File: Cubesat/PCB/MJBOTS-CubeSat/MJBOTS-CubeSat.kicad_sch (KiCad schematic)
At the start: 19 parts, among them J1 Display, J10 MOTOR3-XT30, J12 MOTOR3, J2 MPU 6050, J3 Pi_GPIO, J4 CAN, J5 MOTOR1, J6 MOTOR2, J7 INPUT-XT60, J8 MOTOR1-XT30, J9 MOTOR2-XT30, U1 LM2596S

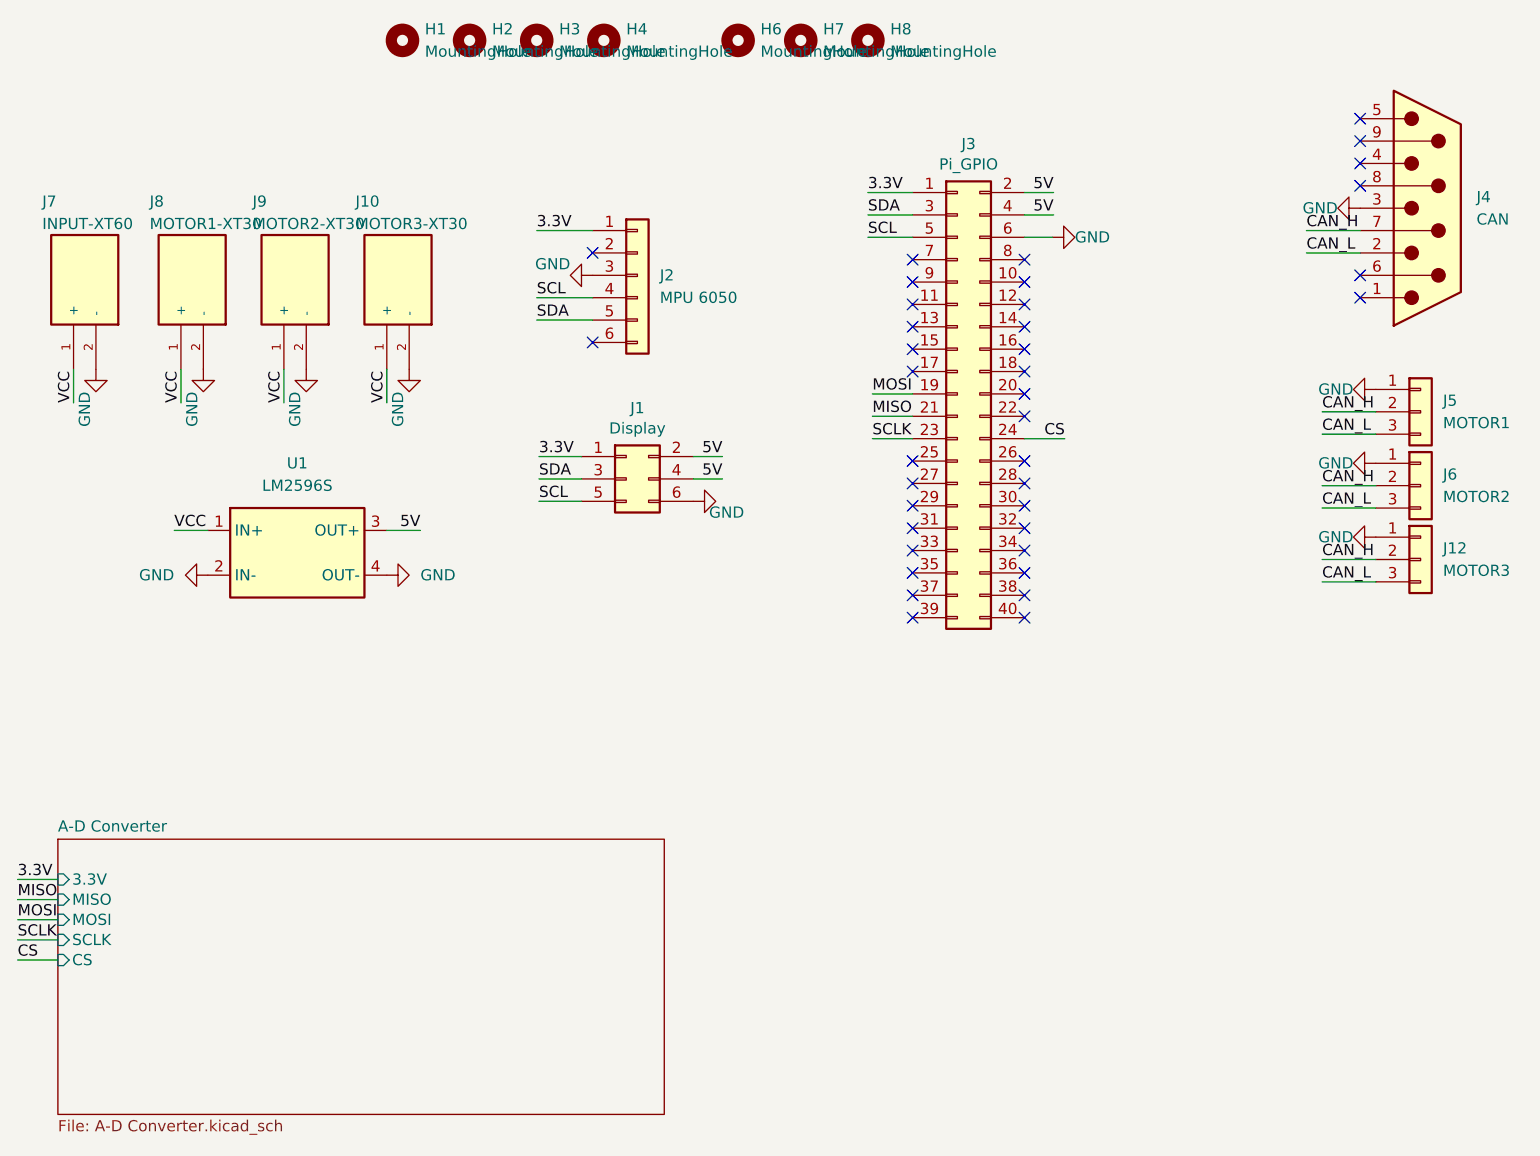
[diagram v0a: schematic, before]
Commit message: Final Updates "HOPEFULLY"
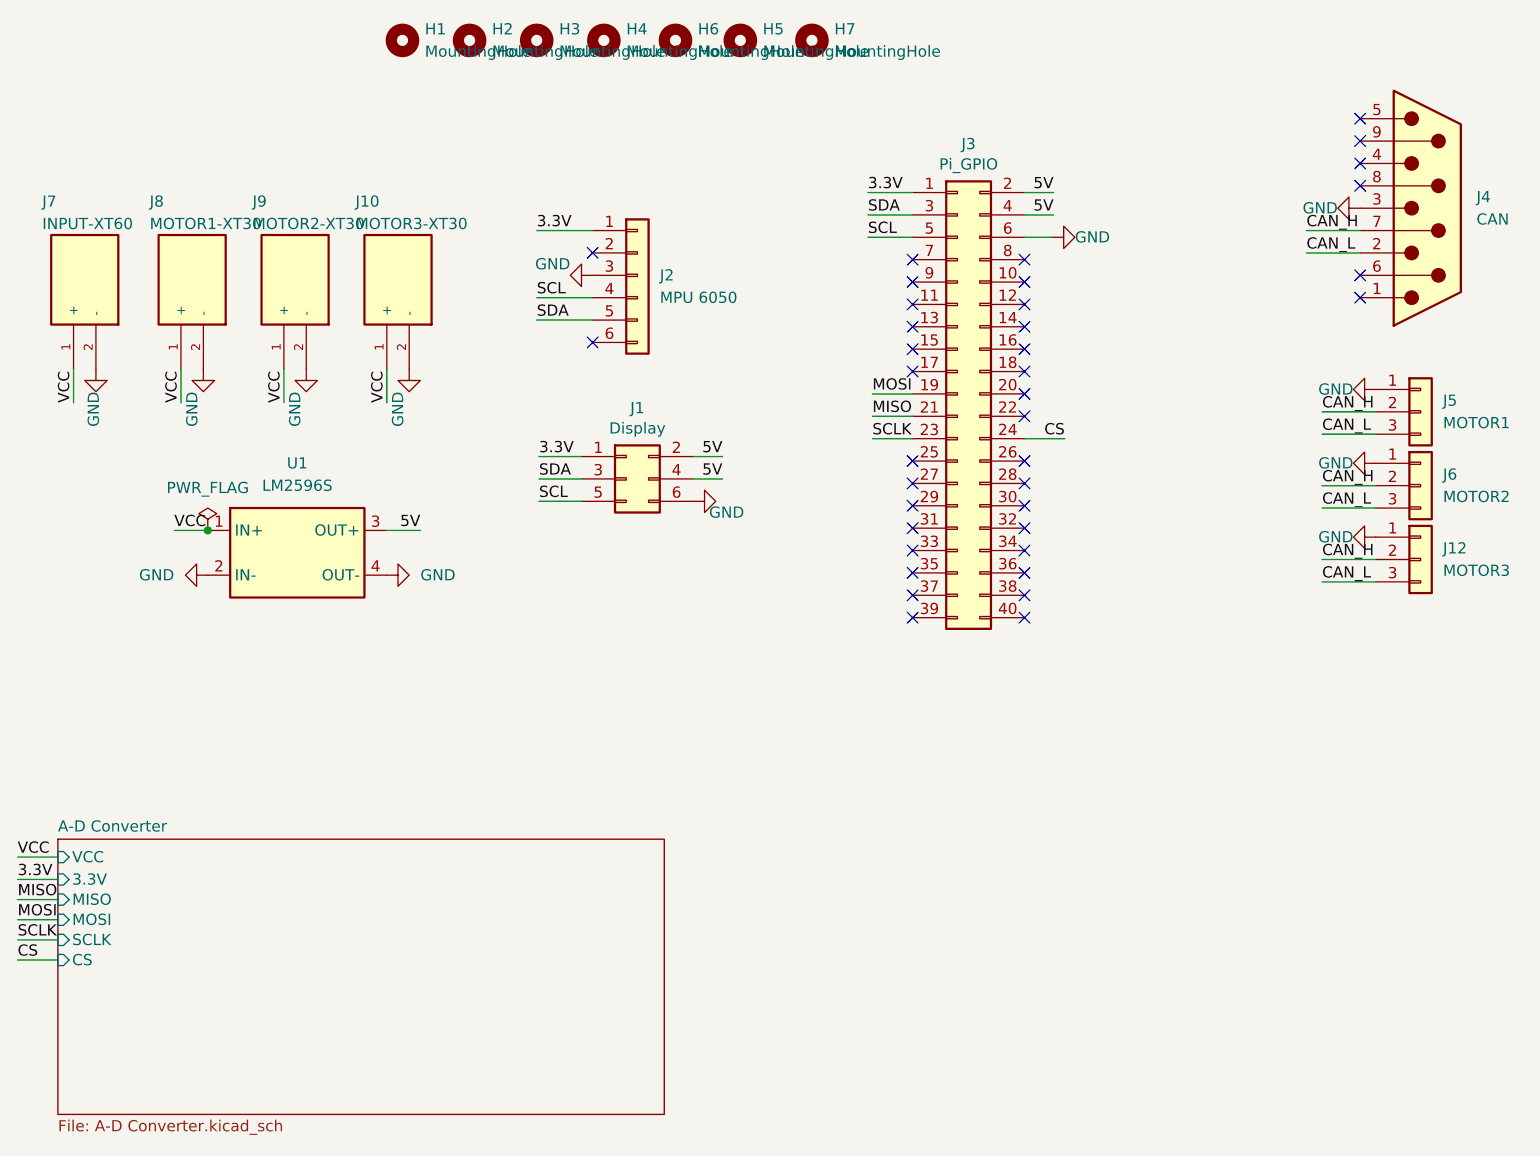
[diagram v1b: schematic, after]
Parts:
- removed H8: MountingHole, MountingHole:MountingHole_2.5mm, symbol Mechanical:MountingHole
- added H5: MountingHole, MountingHole:MountingHole_2.5mm, symbol Mechanical:MountingHole
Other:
- sheet A-D Converter ports: added VCC; removed none
- moved on the sheet: H6
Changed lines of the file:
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@@
 (kicad_sch (version 20211123) (generator eeschema)
   (paper "A4")
+  (junction (at 76.962 96.266) (diameter 0) (color 0 0 0 0)
+  )
   (no_connect (at 156.972 98.552))
   (no_connect (at 156.972 65.532))
@@
     (stroke (width 0) (type default) (color 0 0 0 0))
   )
+  (wire (pts (xy 55.372 133.35) (xy 59.944 133.35))
+    (stroke (width 0) (type default) (color 0 0 0 0))
+  )
   (wire (pts (xy 151.892 60.452) (xy 156.972 60.452))
     (stroke (width 0) (type default) (color 0 0 0 0))
@@
     (effects (font (size 1.27 1.27)) (justify left bottom))
   )
+  (label "VCC" (at 55.372 133.35 0)
+    (effects (font (size 1.27 1.27)) (justify left bottom))
+  )
   (label "5V" (at 135.382 90.424 180)
     (effects (font (size 1.27 1.27)) (justify right bottom))
@@
     (effects (font (size 1.27 1.27)) (justify left bottom))
   )
-  (symbol (lib_id "Mechanical:MountingHole") (at 137.16 40.64 0) (unit 1)
-    (in_bom yes) (on_board yes) (fields_autoplaced)
-    (property "Reference" "H6" (id 0) (at 139.7 39.3699 0)
-      (effects (font (size 1.27 1.27)) (justify left))
-    )
-    (property "Value" "MountingHole" (id 1) (at 139.7 41.9099 0)
-      (effects (font (size 1.27 1.27)) (justify left))
-    )
-    (property "Footprint" "MountingHole:MountingHole_2.5mm" (id 2) (at 137.16 40.64 0)
-      (effects (font (size 1.27 1.27)) hide)
-    )
-    (property "Datasheet" "~" (id 3) (at 137.16 40.64 0)
+  (symbol (lib_id "Mechanical:MountingHole") (at 130.048 40.64 0) (unit 1)
+    (in_bom yes) (on_board yes) (fields_autoplaced)
+    (property "Reference" "H6" (id 0) (at 132.588 39.3699 0)
+      (effects (font (size 1.27 1.27)) (justify left))
+    )
+    (property "Value" "MountingHole" (id 1) (at 132.588 41.9099 0)
+      (effects (font (size 1.27 1.27)) (justify left))
+    )
+    (property "Footprint" "MountingHole:MountingHole_2.5mm" (id 2) (at 130.048 40.64 0)
+      (effects (font (size 1.27 1.27)) hide)
+    )
+    (property "Datasheet" "~" (id 3) (at 130.048 40.64 0)
       (effects (font (size 1.27 1.27)) hide)
     )
@@
     (pin "2")
   )
+  (symbol (lib_id "power:PWR_FLAG") (at 76.962 96.266 0) (unit 1)
+    (in_bom yes) (on_board yes) (fields_autoplaced)
+    (property "Reference" "#FLG0102" (id 0) (at 76.962 94.361 0)
+      (effects (font (size 1.27 1.27)) hide)
+    )
+    (property "Value" "PWR_FLAG" (id 1) (at 76.962 91.44 0))
+    (property "Footprint" "" (id 2) (at 76.962 96.266 0)
+      (effects (font (size 1.27 1.27)) hide)
+    )
+    (property "Datasheet" "~" (id 3) (at 76.962 96.266 0)
+      (effects (font (size 1.27 1.27)) hide)
+    )
+    (pin "1")
+  )
   (symbol (lib_id "power:GND") (at 76.454 77.978 0) (unit 1)
     (in_bom yes) (on_board yes)
@@
       (effects (font (size 1.27 1.27)) hide)
     )
-    (property "Value" "GND" (id 1) (at 62.992 80.518 90)
+    (property "Value" "GND" (id 1) (at 64.008 80.518 90)
       (effects (font (size 1.27 1.27)) (justify right))
     )
@@
     )
   )
+  (symbol (lib_id "Mechanical:MountingHole") (at 145.542 40.64 0) (unit 1)
+    (in_bom yes) (on_board yes) (fields_autoplaced)
+    (property "Reference" "H7" (id 0) (at 148.082 39.3699 0)
+      (effects (font (size 1.27 1.27)) (justify left))
+    )
+    (property "Value" "MountingHole" (id 1) (at 148.082 41.9099 0)
+      (effects (font (size 1.27 1.27)) (justify left))
+    )
+    (property "Footprint" "MountingHole:MountingHole_2.5mm" (id 2) (at 145.542 40.64 0)
+      (effects (font (size 1.27 1.27)) hide)
+    )
+    (property "Datasheet" "~" (id 3) (at 145.542 40.64 0)
+      (effects (font (size 1.27 1.27)) hide)
+    )
+  )
   (symbol (lib_id "24V_Li_batt:Conn_01x03") (at 214.63 91.186 0) (unit 1)
     (in_bom yes) (on_board yes) (fields_autoplaced)
@@
     (pin "1")
   )
-  (symbol (lib_id "Mechanical:MountingHole") (at 144.272 40.64 0) (unit 1)
-    (in_bom yes) (on_board yes) (fields_autoplaced)
-    (property "Reference" "H7" (id 0) (at 146.812 39.3699 0)
-      (effects (font (size 1.27 1.27)) (justify left))
-    )
-    (property "Value" "MountingHole" (id 1) (at 146.812 41.9099 0)
-      (effects (font (size 1.27 1.27)) (justify left))
-    )
-    (property "Footprint" "MountingHole:MountingHole_2.5mm" (id 2) (at 144.272 40.64 0)
-      (effects (font (size 1.27 1.27)) hide)
-    )
-    (property "Datasheet" "~" (id 3) (at 144.272 40.64 0)
+  (symbol (lib_id "Mechanical:MountingHole") (at 137.414 40.64 0) (unit 1)
+    (in_bom yes) (on_board yes) (fields_autoplaced)
+    (property "Reference" "H5" (id 0) (at 139.954 39.3699 0)
+      (effects (font (size 1.27 1.27)) (justify left))
+    )
+    (property "Value" "MountingHole" (id 1) (at 139.954 41.9099 0)
+      (effects (font (size 1.27 1.27)) (justify left))
+    )
+    (property "Footprint" "MountingHole:MountingHole_2.5mm" (id 2) (at 137.414 40.64 0)
+      (effects (font (size 1.27 1.27)) hide)
+    )
+    (property "Datasheet" "~" (id 3) (at 137.414 40.64 0)
       (effects (font (size 1.27 1.27)) hide)
     )
@@
     (pin "5")
     (pin "6")
-  )
-  (symbol (lib_id "Mechanical:MountingHole") (at 151.892 40.64 0) (unit 1)
-    (in_bom yes) (on_board yes) (fields_autoplaced)
-    (property "Reference" "H8" (id 0) (at 154.432 39.3699 0)
-      (effects (font (size 1.27 1.27)) (justify left))
-    )
-    (property "Value" "MountingHole" (id 1) (at 154.432 41.9099 0)
-      (effects (font (size 1.27 1.27)) (justify left))
-    )
-    (property "Footprint" "MountingHole:MountingHole_2.5mm" (id 2) (at 151.892 40.64 0)
-      (effects (font (size 1.27 1.27)) hide)
-    )
-    (property "Datasheet" "~" (id 3) (at 151.892 40.64 0)
-      (effects (font (size 1.27 1.27)) hide)
-    )
   )
   (symbol (lib_id "Connector_Generic:Conn_02x20_Odd_Even") (at 162.052 80.772 0) (unit 1)
@@
       (effects (font (size 1.27 1.27)) (justify left))
     )
+    (pin "VCC" input (at 59.944 133.35 180)
+      (effects (font (size 1.27 1.27)) (justify left))
+    )
   )
   (sheet_instances
@@
       (reference "#FLG0101") (unit 1) (value "PWR_FLAG") (footprint "")
     )
+    (path "/353dcdab-295b-4884-b99f-346e0d932e58"
+      (reference "#FLG0102") (unit 1) (value "PWR_FLAG") (footprint "")
+    )
     (path "/e720ff28-7203-4205-97be-458b252c135b"
       (reference "#PWR0101") (unit 1) (value "GND") (footprint "")
@@
       (reference "#PWR0115") (unit 1) (value "GND") (footprint "")
     )
+    (path "/f4ba3478-2c95-496a-9c27-457b9411cacb/508cb951-553a-42aa-98fb-8fbae1b6eb7d"
+      (reference "#PWR0116") (unit 1) (value "GND") (footprint "")
+    )
     (path "/c125495c-82f3-42db-8b42-bf22cefa9f79"
       (reference "H1") (unit 1) (value "MountingHole") (footprint "MountingHole:MountingHole_2.5mm")
@@
       (reference "H4") (unit 1) (value "MountingHole") (footprint "MountingHole:MountingHole_2.5mm")
     )
+    (path "/b6794ca9-37d2-4959-ad5a-b6899fdc0e43"
+      (reference "H5") (unit 1) (value "MountingHole") (footprint "MountingHole:MountingHole_2.5mm")
+    )
     (path "/20538c33-4b7b-4c78-9d68-b98cd9361aea"
       (reference "H6") (unit 1) (value "MountingHole") (footprint "MountingHole:MountingHole_2.5mm")
     )
-    (path "/ab523916-fa2e-4753-93b6-47b9afdd276b"
+    (path "/6ea51669-04b2-4d14-bdca-acba8fa3ebde"
       (reference "H7") (unit 1) (value "MountingHole") (footprint "MountingHole:MountingHole_2.5mm")
-    )
-    (path "/da6f9729-f218-46e4-b198-41468c381a9f"
-      (reference "H8") (unit 1) (value "MountingHole") (footprint "MountingHole:MountingHole_2.5mm")
     )
     (path "/d5de051d-d0f2-40e1-9291-05aae056795f"
@@
       (reference "J10") (unit 1) (value "MOTOR3-XT30") (footprint "cube:XT30PWM")
     )
-    (path "/f4ba3478-2c95-496a-9c27-457b9411cacb/beb10ef3-eb97-446c-b630-ee80bacfd364"
-      (reference "J11") (unit 1) (value "JST-BATT") (footprint "Connector_PinHeader_2.54mm:PinHeader_1x04_P2.54mm_Vertical")
-    )
     (path "/fe307aa7-3d5b-431f-be0c-bc0fbe8002f0"
       (reference "J12") (unit 1) (value "MOTOR3") (footprint "Connector_PinHeader_2.54mm:PinHeader_1x03_P2.54mm_Vertical")
     )
+    (path "/f4ba3478-2c95-496a-9c27-457b9411cacb/15aa997a-aa5a-45f8-8a4d-cd6b3343a02a"
+      (reference "R1") (unit 1) (value "2k") (footprint "Resistor_SMD:R_0805_2012Metric_Pad1.20x1.40mm_HandSolder")
+    )
+    (path "/f4ba3478-2c95-496a-9c27-457b9411cacb/ba176358-80f6-4f7a-9db6-3bd603290649"
+      (reference "R2") (unit 1) (value "1k") (footprint "Resistor_SMD:R_0805_2012Metric_Pad1.20x1.40mm_HandSolder")
+    )
     (path "/56f63a98-abd0-410c-bb66-f75481e1c26f"
